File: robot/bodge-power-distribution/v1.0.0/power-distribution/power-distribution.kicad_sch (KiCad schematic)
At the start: 14 parts, among them J1 Conn_01x02, SW1 CF-LD-1DC4-AR2W

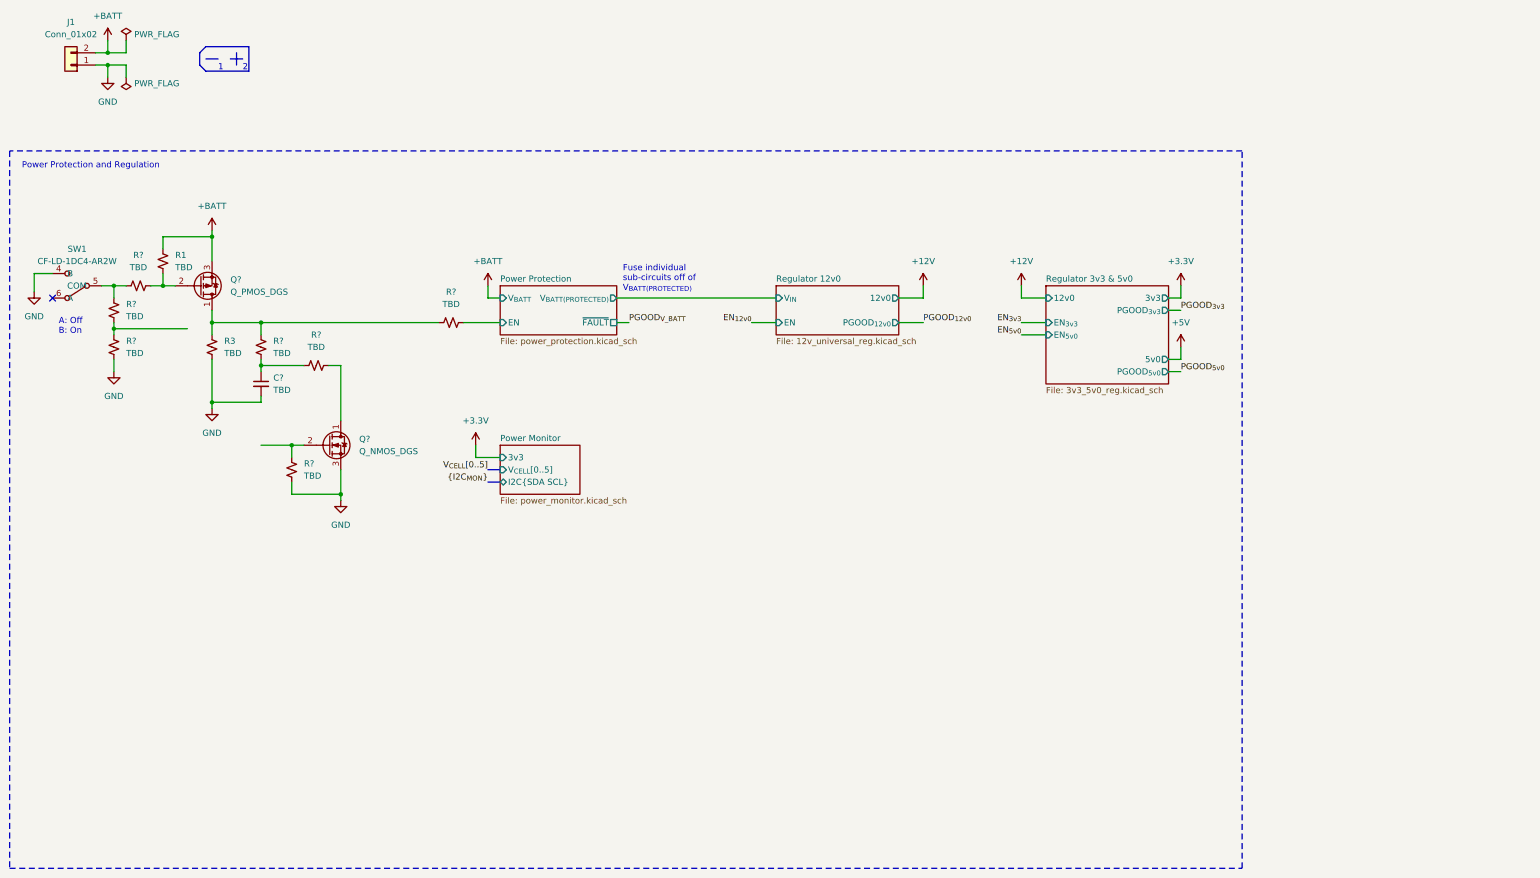
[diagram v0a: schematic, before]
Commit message: Sync
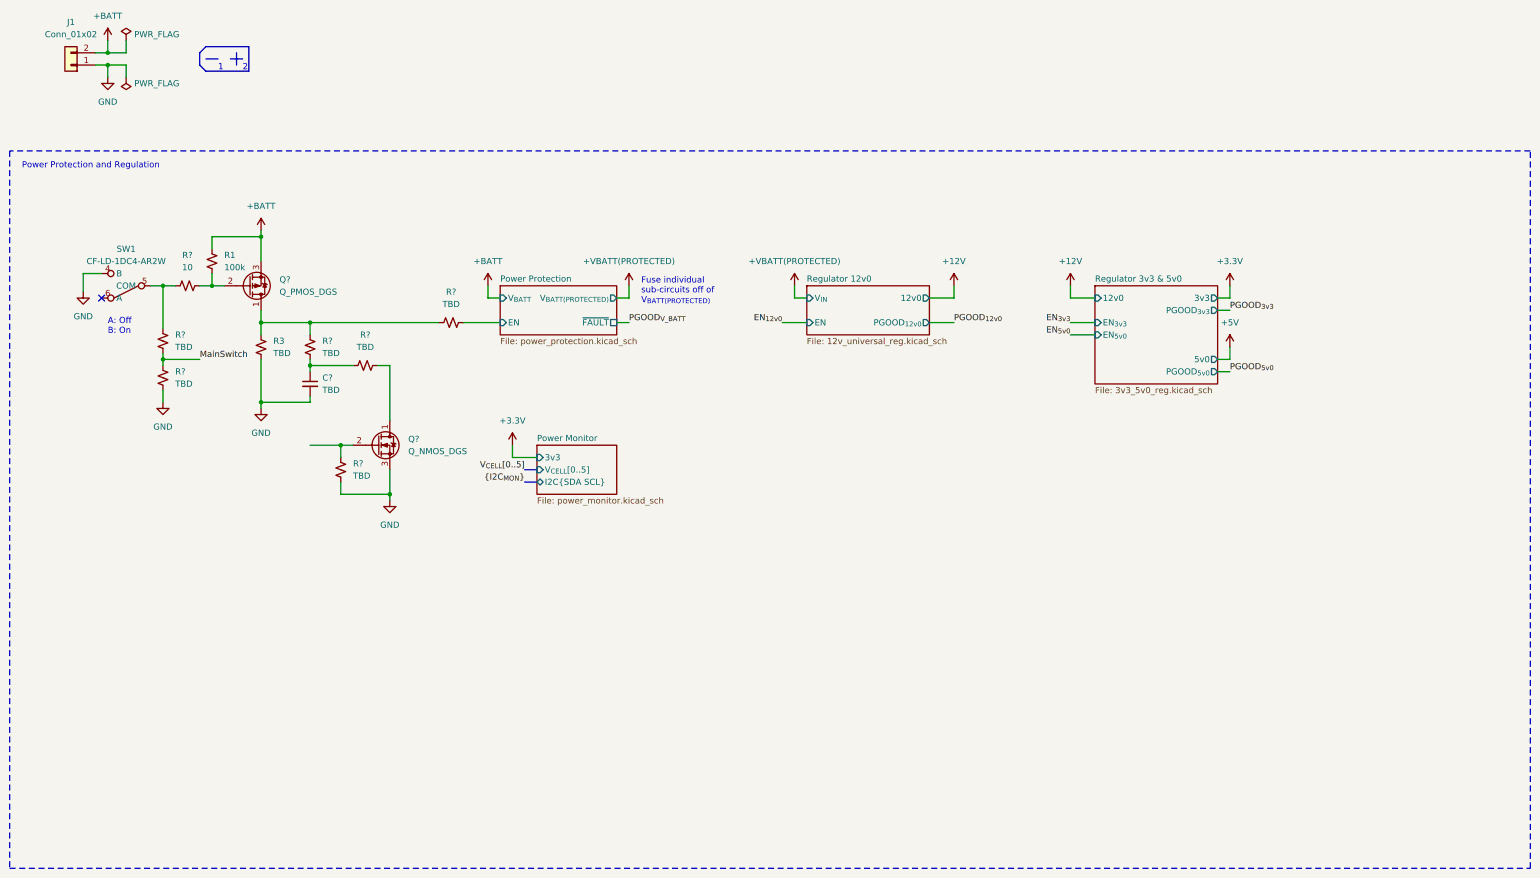
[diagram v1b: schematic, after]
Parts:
- R1: value TBD -> 100k
- R?: value TBD -> 10
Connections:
- net MainSwitch: now reaches R?.1, R?.2
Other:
- moved on the sheet: C?, Q?, R1, R3, R?, SW1
